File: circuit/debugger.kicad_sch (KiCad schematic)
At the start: 1 part

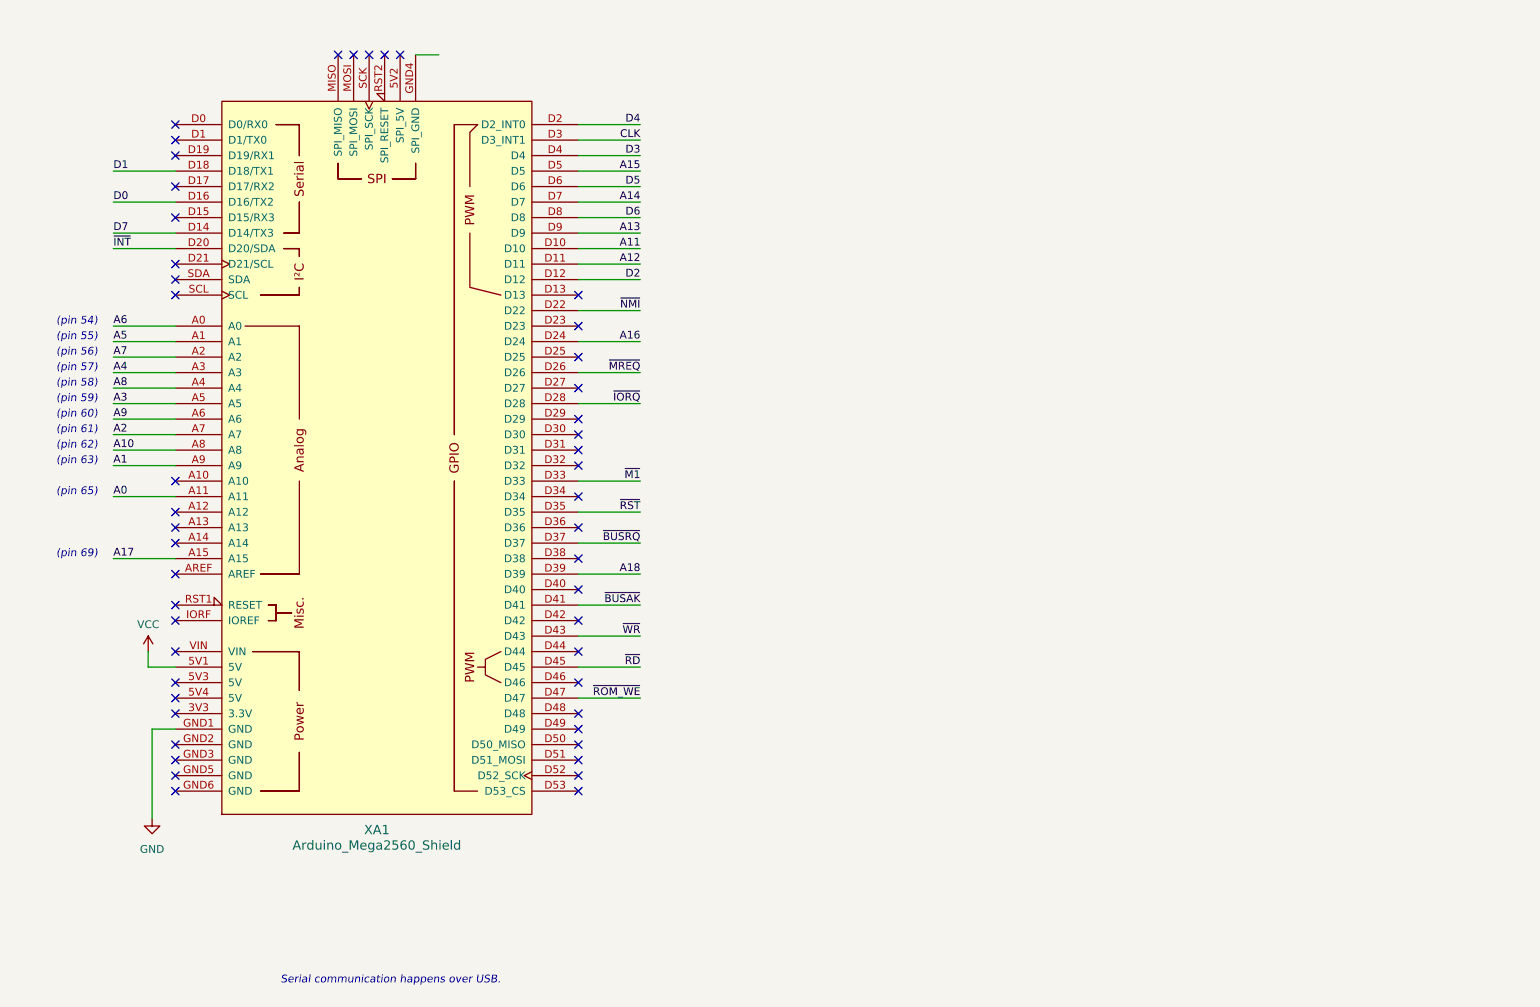
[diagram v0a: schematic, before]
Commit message: .
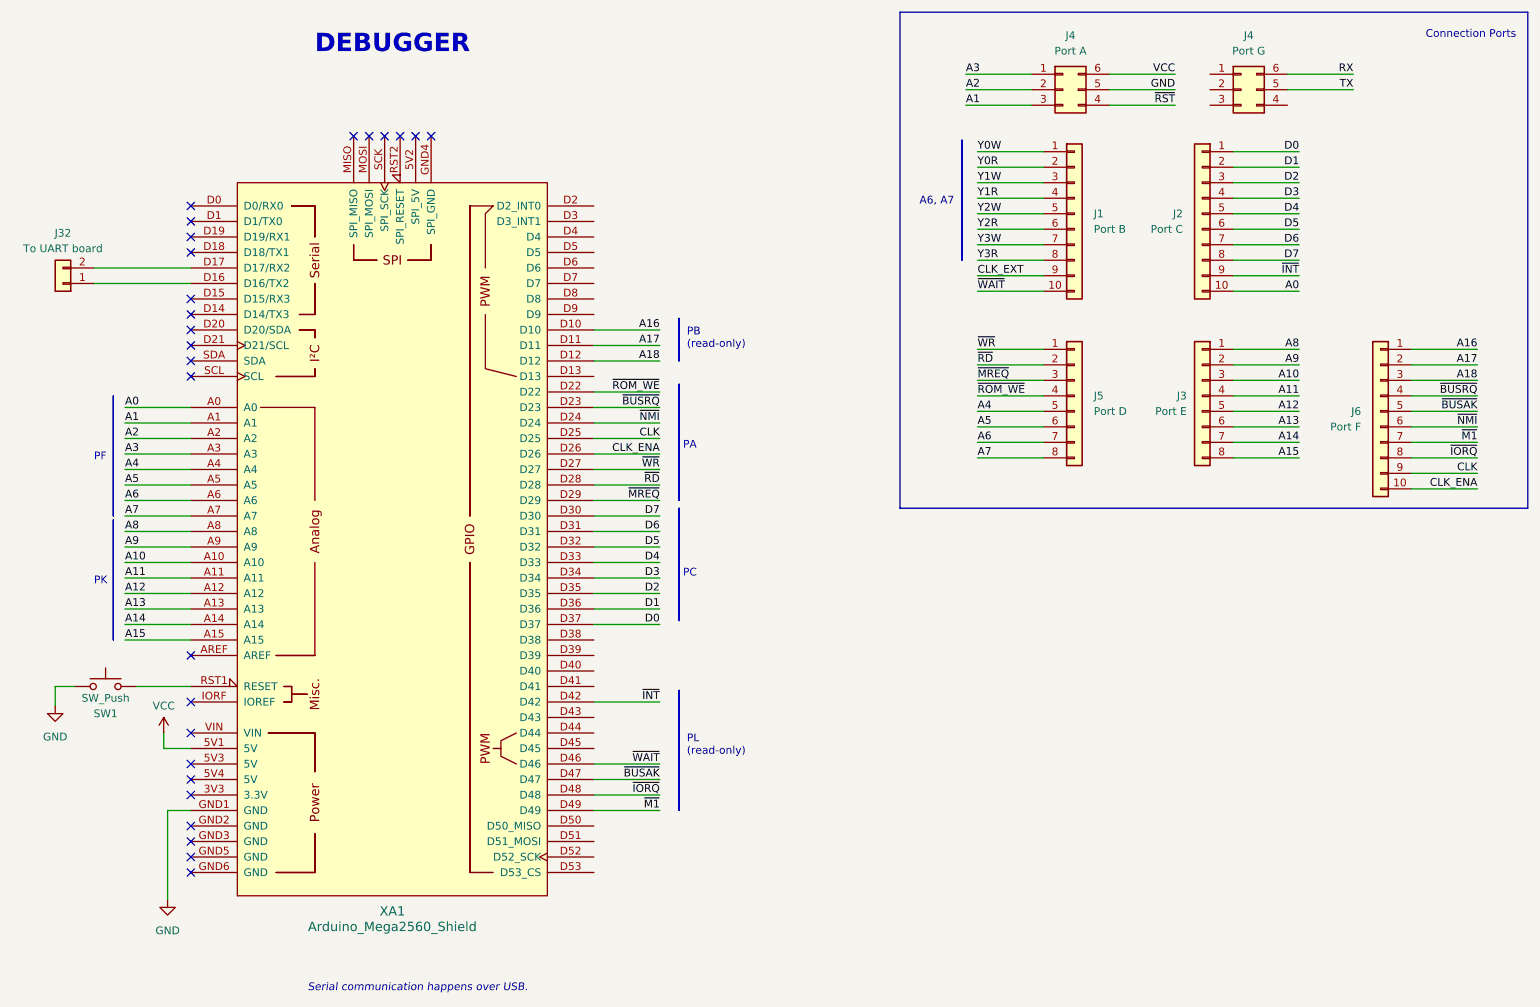
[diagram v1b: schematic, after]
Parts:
- added J1: Port B, symbol Connector_Generic:Conn_01x10
- added J2: Port C, symbol Connector_Generic:Conn_01x10
- added J3: Port E, symbol Connector_Generic:Conn_01x08
- added J32: To UART board, symbol Connector_Generic:Conn_01x02
- added J4: Port A, symbol Connector_Generic:Conn_02x03_Counter_Clockwise
- added J4: Port G, symbol Connector_Generic:Conn_02x03_Counter_Clockwise
- added J5: Port D, symbol Connector_Generic:Conn_01x08
- added J6: Port F, symbol Connector_Generic:Conn_01x10
- added SW1: SW_Push, symbol Switch:SW_Push
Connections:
- net A0: now also XA1.A0, J2.10 (Pin_10); no longer XA1.A11
- net A1: now also XA1.A1, J4.3 (Pin_3); no longer XA1.A9
- net A10: now also XA1.A10, J3.3 (Pin_3); no longer XA1.A8
- net A11: now also XA1.A11, J3.4 (Pin_4); no longer XA1.D10
- net A12: now also XA1.A12, J3.5 (Pin_5); no longer XA1.D11
- net A13: now also XA1.A13, J3.6 (Pin_6); no longer XA1.D9
- net A14: now also XA1.A14, J3.7 (Pin_7); no longer XA1.D7
- net A15: now also XA1.A15, J3.8 (Pin_8); no longer XA1.D5
- net A16: now also XA1.D10, J6.1 (Pin_1); no longer XA1.D24
- net A17: now also XA1.D11, J6.2 (Pin_2); no longer XA1.A15
- net A18: now also XA1.D12, J6.3 (Pin_3); no longer XA1.D39
- net A2: now also XA1.A2, J4.2 (Pin_2); no longer XA1.A7
- net A3: now also XA1.A3, J4.1 (Pin_1); no longer XA1.A5
- net A4: now also XA1.A4, J5.5 (Pin_5); no longer XA1.A3
- net A5: now also XA1.A5, J5.6 (Pin_6); no longer XA1.A1
- net A6: now also XA1.A6, J5.7 (Pin_7); no longer XA1.A0
- net A7: now also XA1.A7, J5.8 (Pin_8); no longer XA1.A2
- net A8: now also XA1.A8, J3.1 (Pin_1); no longer XA1.A4
- net A9: now also XA1.A9, J3.2 (Pin_2); no longer XA1.A6
- net CLK: now also XA1.D25, J6.9 (Pin_9); no longer XA1.D3 (D3_INT1)
- net D0: now also XA1.D37, J2.1 (Pin_1); no longer XA1.D16 (D16/TX2)
- net D1: now also XA1.D36, J2.2 (Pin_2); no longer XA1.D18 (D18/TX1)
- net D2: now also XA1.D35, J2.3 (Pin_3); no longer XA1.D12
- net D3: now also XA1.D34, J2.4 (Pin_4); no longer XA1.D4
- net D4: now also XA1.D33, J2.5 (Pin_5); no longer XA1.D2 (D2_INT0)
- net D5: now also XA1.D32, J2.6 (Pin_6); no longer XA1.D6
- net D6: now also XA1.D31, J2.7 (Pin_7); no longer XA1.D8
- net D7: now also XA1.D30, J2.8 (Pin_8); no longer XA1.D14 (D14/TX3)
- net GND: now also J4.5 (Pin_5), SW1.1
- net VCC: now also J4.6 (Pin_6)
- net ~{BUSAK}: now also XA1.D47, J6.5 (Pin_5); no longer XA1.D41
- net ~{BUSRQ}: now also XA1.D23, J6.4 (Pin_4); no longer XA1.D37
- net ~{INT}: now also XA1.D42, J2.9 (Pin_9); no longer XA1.D20 (D20/SDA)
- net ~{IORQ}: now also XA1.D48, J6.8 (Pin_8); no longer XA1.D28
- net ~{M1}: now also XA1.D49, J6.7 (Pin_7); no longer XA1.D33
- net ~{MREQ}: now also XA1.D29, J5.3 (Pin_3); no longer XA1.D26
- net ~{NMI}: now also XA1.D24, J6.6 (Pin_6); no longer XA1.D22
- net ~{RD}: now also XA1.D28, J5.2 (Pin_2); no longer XA1.D45
- net ~{ROM_WE}: now also XA1.D22, J5.4 (Pin_4); no longer XA1.D47
- net ~{RST}: now also J4.4 (Pin_4); no longer XA1.D35
- net ~{WR}: now also XA1.D27, J5.1 (Pin_1); no longer XA1.D43
- net at XA1.D17 (D17/RX2): now also J32.2 (Pin_2)
- net ~{WAIT}: now reaches XA1.D46
- net ~{WAIT}: now also J1.10 (Pin_10)
- net at XA1.RST1 (RESET): now also SW1.2
- new net: J32.1 (Pin_1), XA1.D16 (D16/TX2)
- new net CLK_ENA: J6.10 (Pin_10), XA1.D26
- new net CLK_EXT: J1.9 (Pin_9)
- new net RX: J4.6 (Pin_6)
- new net TX: J4.5 (Pin_5)
- new net Y0R: J1.2 (Pin_2)
- new net Y0W: J1.1 (Pin_1)
- new net Y1R: J1.4 (Pin_4)
- new net Y1W: J1.3 (Pin_3)
- new net Y2R: J1.6 (Pin_6)
- new net Y2W: J1.5 (Pin_5)
- new net Y3R: J1.8 (Pin_8)
- new net Y3W: J1.7 (Pin_7)
- no-connect marks 49 -> 26
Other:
- note added: "A6, A7"
- note added: "Connection Ports"
- note added: "DEBUGGER"
- note added: "PA"
- note added: "PB (read-only)"
- note added: "PC"
- note added: "PF"
- note added: "PK"
- note added: "PL (read-only)"
- note removed: "(pin 54)"
- note removed: "(pin 55)"
- note removed: "(pin 56)"
- note removed: "(pin 57)"
- note removed: "(pin 58)"
- note removed: "(pin 59)"
- note removed: "(pin 60)"
- note removed: "(pin 61)"
- note removed: "(pin 62)"
- note removed: "(pin 63)"
- note removed: "(pin 65)"
- note removed: "(pin 69)"
- moved on the sheet: XA1
